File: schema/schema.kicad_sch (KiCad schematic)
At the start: 2 parts, among them J1 Conn_01x14_Pin, U1 ATmega8A-P

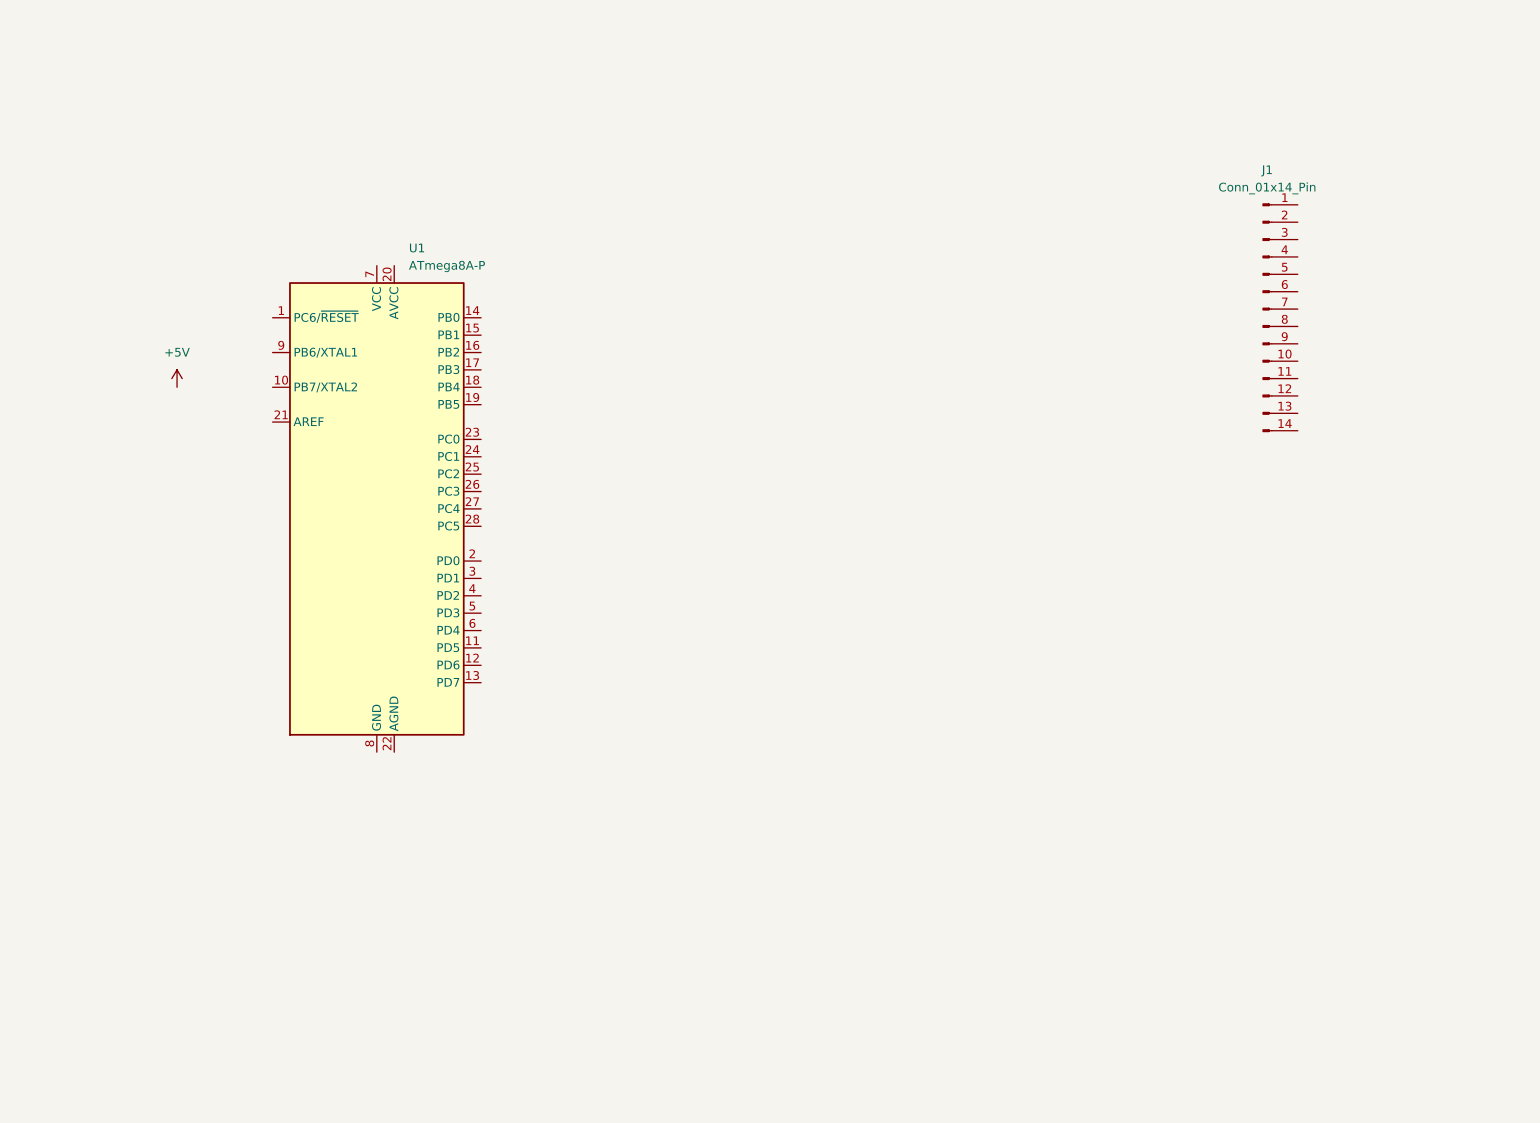
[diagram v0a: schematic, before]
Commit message: wip
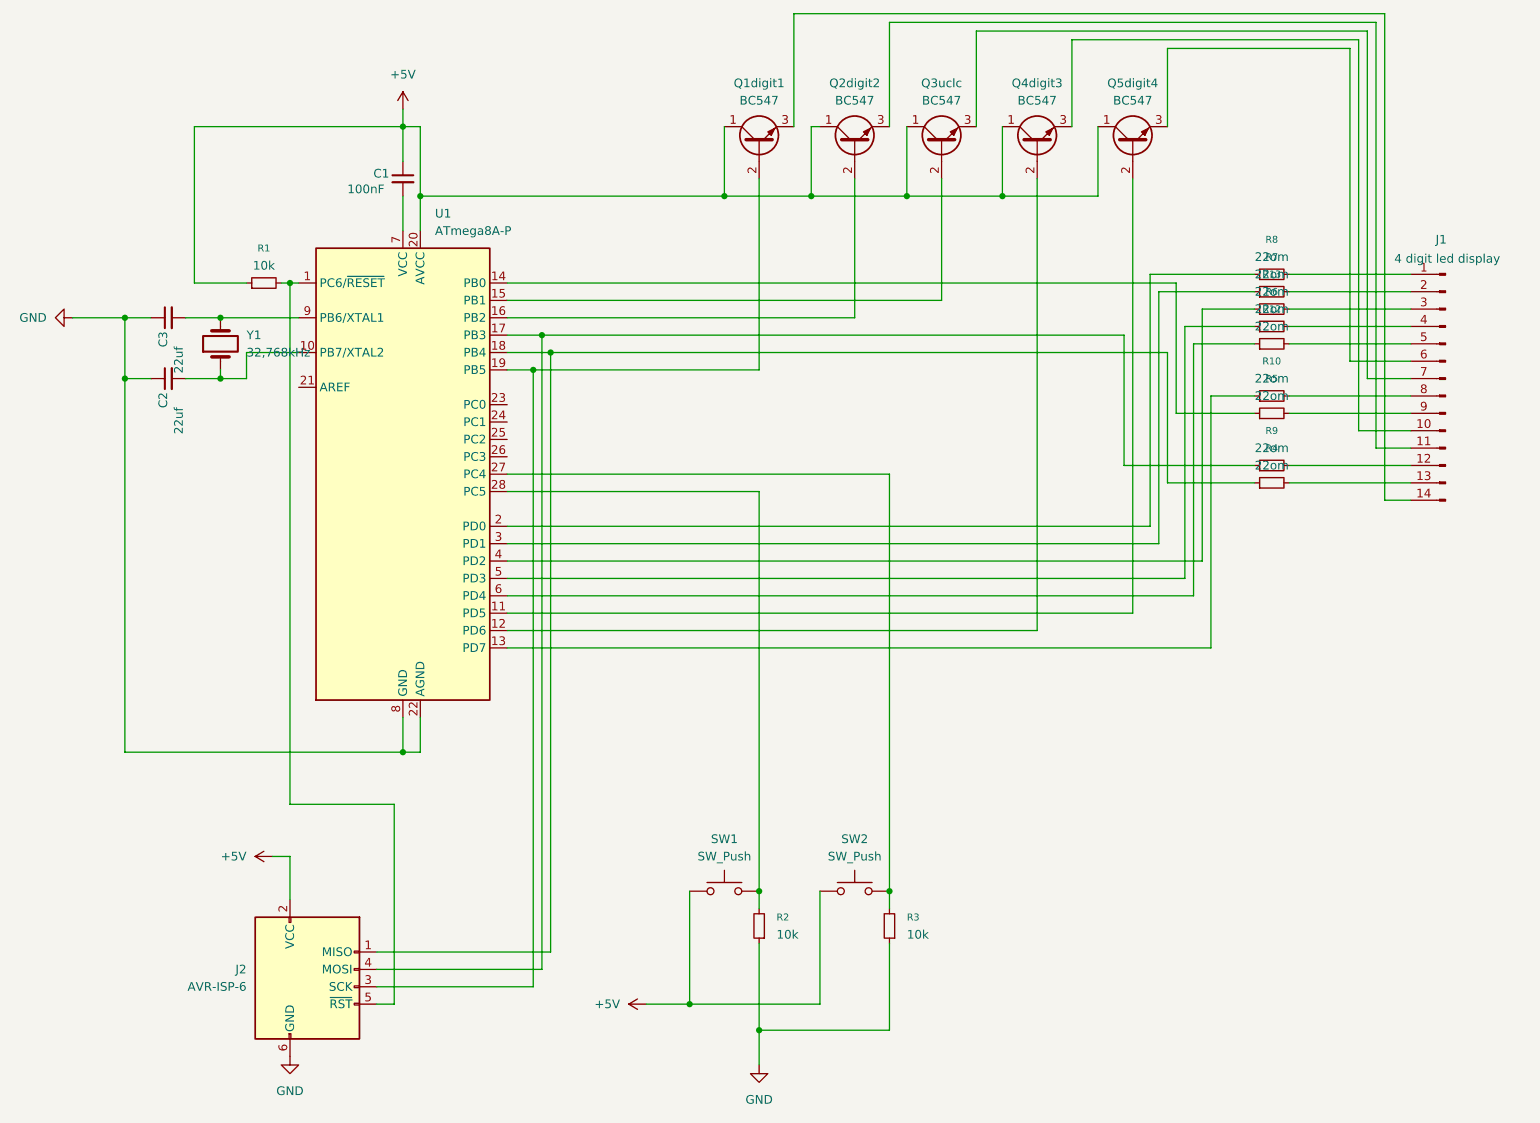
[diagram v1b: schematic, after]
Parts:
- added C1: 100nF, symbol Device:C_Small
- added C2, C3: 22uf, symbol Device:C_Small
- added J2: AVR-ISP-6, symbol Connector:AVR-ISP-6
- added Q1digit1, Q2digit2, Q3uclc, Q4digit3, Q5digit4: BC547, Package_TO_SOT_THT:TO-92_Inline, symbol Transistor_BJT:BC547
- added R1, R2, R3: 10k, symbol Device:R_Small
- added R10, R12, R13, R4, R5, R6, R7, R8, R9: 22om, symbol Device:R_Small
- added SW1, SW2: SW_Push, symbol Switch:SW_Push
- added Y1: 32,768kHz, symbol Device:Crystal
- J1: value Conn_01x14_Pin -> 4 digit led display
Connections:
- net +5V: now also U1.20 (AVCC), C1.1, J2.2 (VCC), Q1digit1.1 (C), Q2digit2.1 (C), Q3uclc.1 (C), Q4digit3.1 (C), Q5digit4.1 (C), R1.1, SW1.1, SW2.1
- net at U1.1 (PC6/~{RESET}): now also J2.5 (~{RST}), R1.2
- net at U1.10 (PB7/XTAL2): now also C2.2, Y1.1
- net at U1.11 (PD5): now also Q5digit4.2 (B)
- net at U1.12 (PD6): now also Q4digit3.2 (B)
- net at U1.13 (PD7): now also R10.1
- net at U1.14 (PB0): now also R5.1
- net at U1.15 (PB1): now also Q3uclc.2 (B)
- net at U1.16 (PB2): now also Q2digit2.2 (B)
- net at U1.17 (PB3): now also J2.4 (MOSI), R9.1
- net at U1.18 (PB4): now also J2.1 (MISO), R4.1
- net at U1.19 (PB5): now also J2.3 (SCK), Q1digit1.2 (B)
- net at U1.2 (PD0): now also R8.1
- net GND: now reaches U1.22 (AGND)
- net GND: now also U1.8 (GND), C2.1, C3.1, J2.6 (GND), R2.1, R3.1
- net at U1.27 (PC4): now also R3.2, SW2.2
- net at U1.28 (PC5): now also R2.2, SW1.2
- net at U1.3 (PD1): now also R7.1
- net at U1.4 (PD2): now also R13.1
- net at U1.5 (PD3): now also R6.1
- net at U1.6 (PD4): now also R12.1
- net at U1.7 (VCC): now also C1.2
- net at U1.9 (PB6/XTAL1): now also C3.2, Y1.2
- net at J1.1 (Pin_1): now also R8.2
- net at J1.10 (Pin_10): now also Q4digit3.3 (E)
- net at J1.11 (Pin_11): now also Q2digit2.3 (E)
- net at J1.12 (Pin_12): now also R9.2
- net at J1.13 (Pin_13): now also R4.2
- net at J1.14 (Pin_14): now also Q1digit1.3 (E)
- net at J1.2 (Pin_2): now also R7.2
- net at J1.3 (Pin_3): now also R13.2
- net at J1.4 (Pin_4): now also R6.2
- net at J1.5 (Pin_5): now also R12.2
- net at J1.6 (Pin_6): now also Q5digit4.3 (E)
- net at J1.7 (Pin_7): now also Q3uclc.3 (E)
- net at J1.8 (Pin_8): now also R10.2
- net at J1.9 (Pin_9): now also R5.2
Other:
- moved on the sheet: J1, U1
